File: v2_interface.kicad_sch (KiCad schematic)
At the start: 47 parts, among them J10 Power, J11 Vref_Select, J12 AUX_Select, J8 DE9_Socket, J9 DB25_Socket, Q1 2N7002K, Q2 2N7002K, U10 MCP1501-20xCH, U8 MCP4922, U9 MCP3424x-xSL

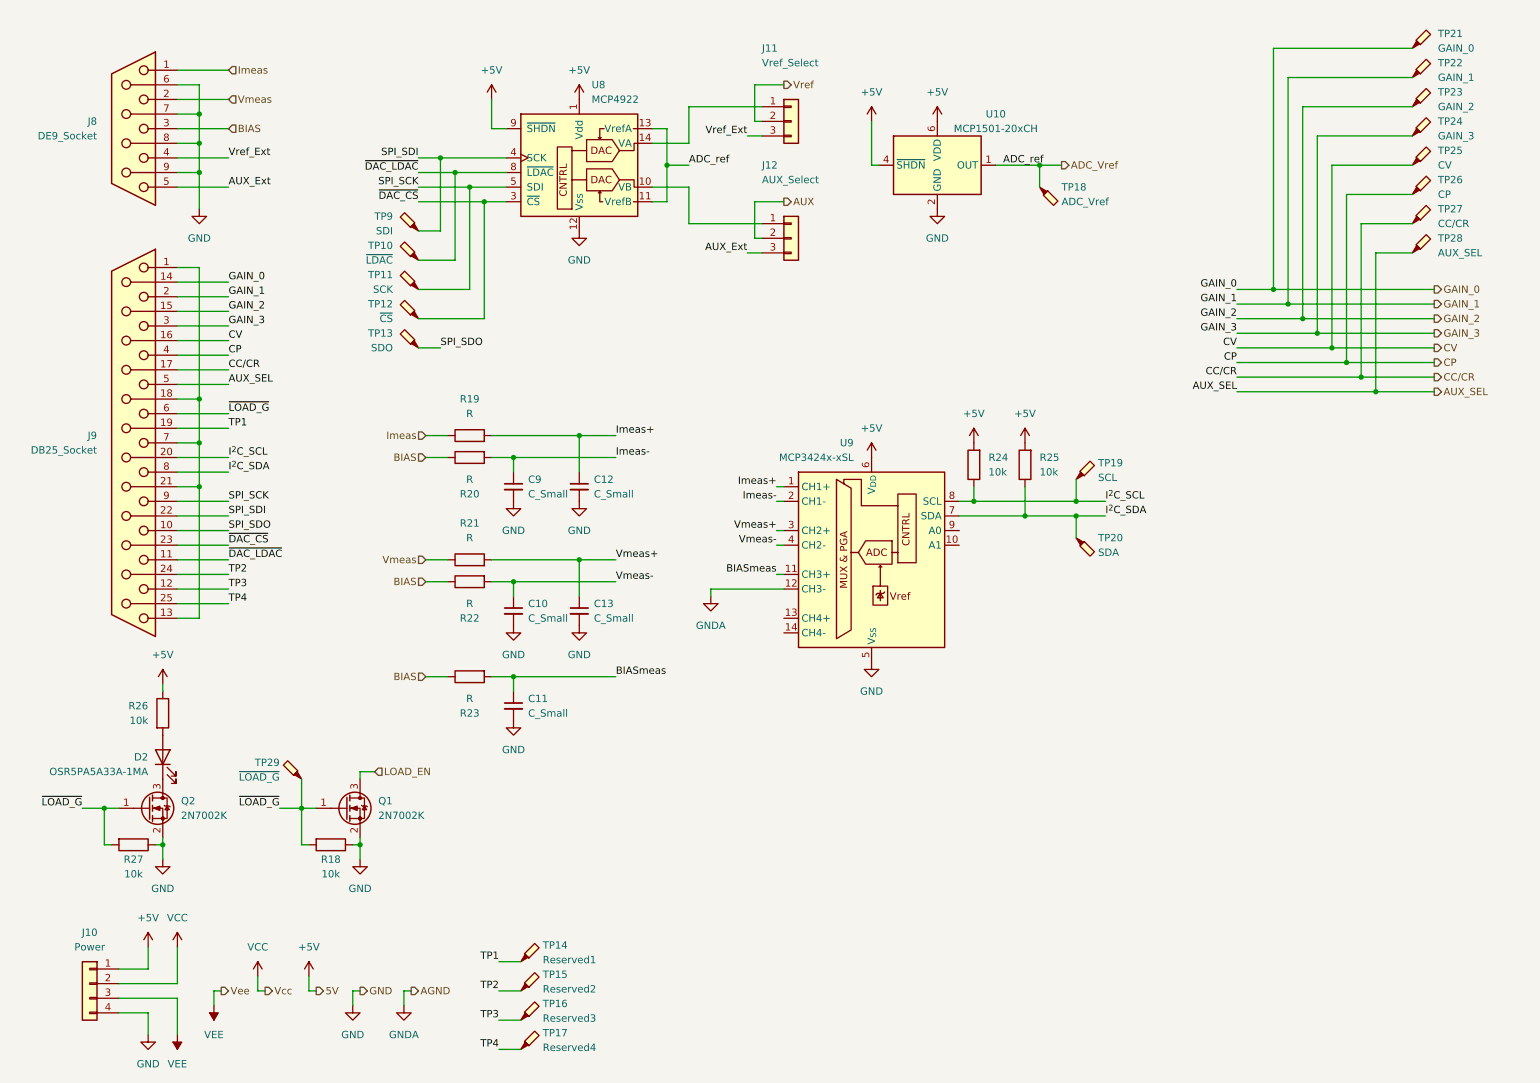
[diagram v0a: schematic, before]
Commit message: sims
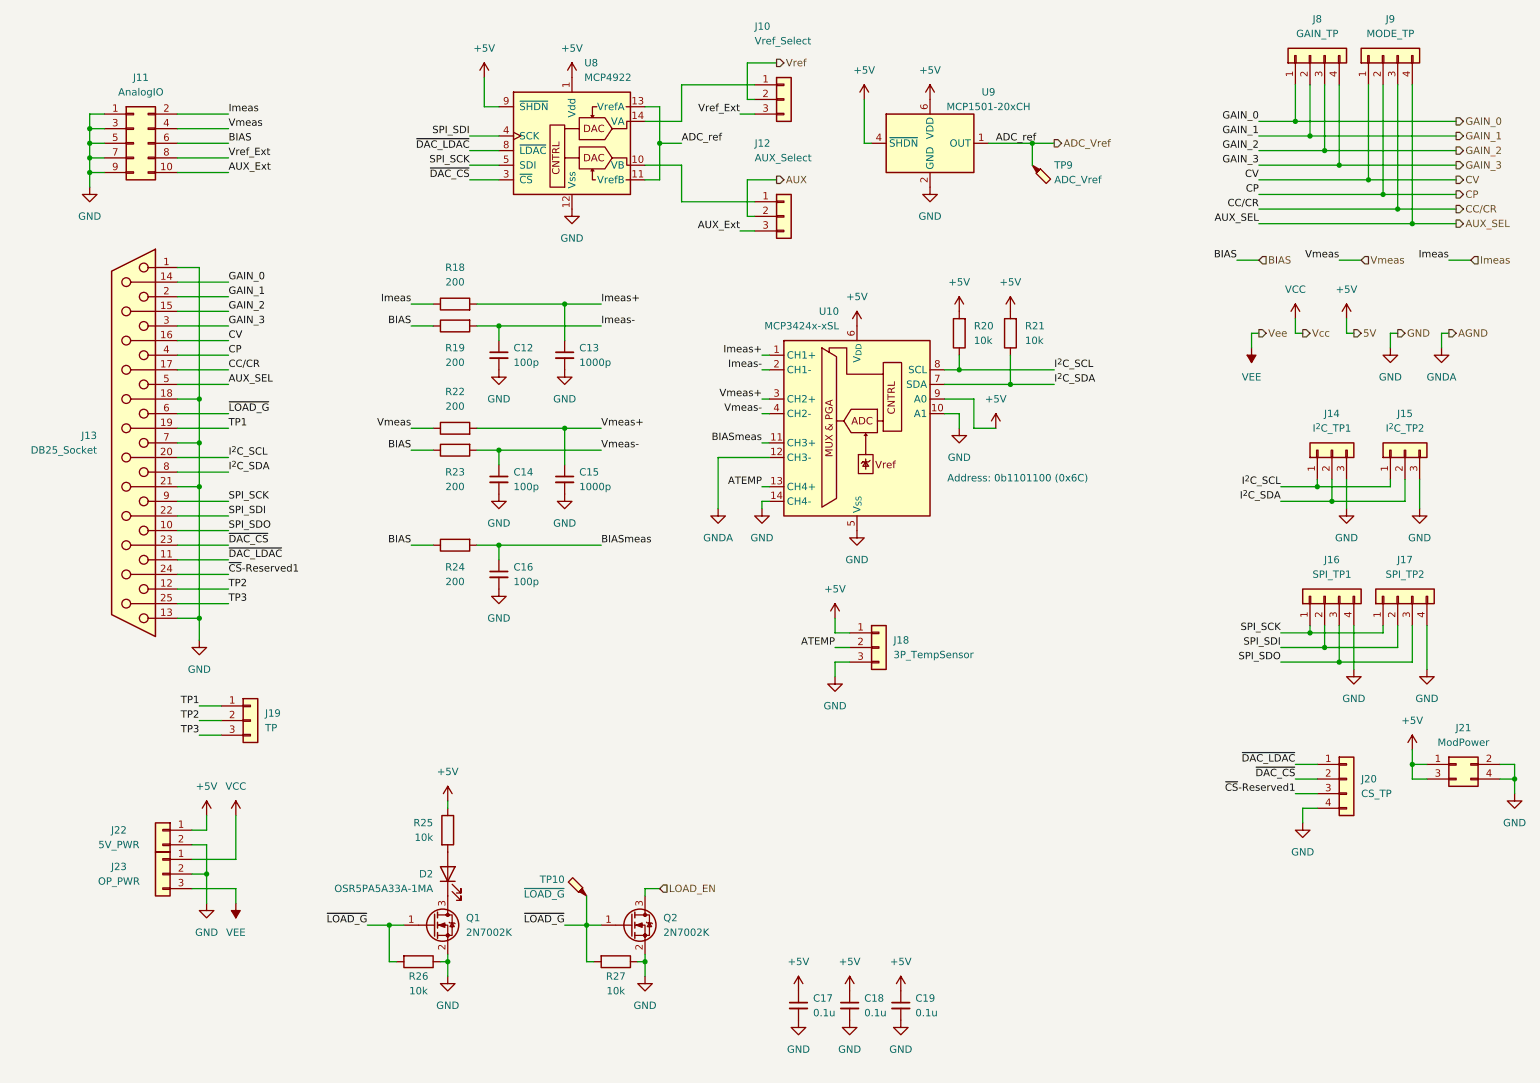
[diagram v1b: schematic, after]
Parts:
- removed J10: Power, AM_Conn_ScrewTerminal:TerminalReceptacle_1x04_P2.54mm, symbol Connector_Generic:Conn_01x04
- removed J8: DE9_Socket, AM_Conn_Dsub:Dsub-9P_2.77mm-2.84mm-8.08mmOffset, symbol Connector:DE9_Socket
- removed TP10: ~{LDAC}, symbol Connector:TestPoint_Probe
- removed TP11: SCK, symbol Connector:TestPoint_Probe
- removed TP12: ~{CS}, symbol Connector:TestPoint_Probe
- removed TP13: SDO, symbol Connector:TestPoint_Probe
- removed TP14: Reserved1, symbol Connector:TestPoint_Probe
- removed TP15: Reserved2, symbol Connector:TestPoint_Probe
- removed TP16: Reserved3, symbol Connector:TestPoint_Probe
- removed TP17: Reserved4, symbol Connector:TestPoint_Probe
- removed TP19: SCL, symbol Connector:TestPoint_Probe
- removed TP20: SDA, symbol Connector:TestPoint_Probe
- removed TP21: GAIN_0, symbol Connector:TestPoint_Probe
- removed TP22: GAIN_1, symbol Connector:TestPoint_Probe
- removed TP23: GAIN_2, symbol Connector:TestPoint_Probe
- removed TP24: GAIN_3, symbol Connector:TestPoint_Probe
- removed TP25: CV, symbol Connector:TestPoint_Probe
- removed TP26: CP, symbol Connector:TestPoint_Probe
- removed TP27: CC/CR, symbol Connector:TestPoint_Probe
- removed TP28: AUX_SEL, symbol Connector:TestPoint_Probe
- removed TP9: SDI, symbol Connector:TestPoint_Probe
- added C17, C18, C19: 0.1u, Capacitor_SMD:C_0603_1608Metric, symbol Device:C_Small
- added J11: AnalogIO, Connector_PinHeader_2.54mm:PinHeader_2x05_P2.54mm_Vertical, symbol Connector_Generic:Conn_02x05_Odd_Even
- added J14: I^{2}C_TP1, Connector_PinHeader_2.54mm:PinHeader_1x03_P2.54mm_Vertical, symbol Connector_Generic:Conn_01x03
- added J15: I^{2}C_TP2, Connector_PinHeader_2.54mm:PinHeader_1x03_P2.54mm_Vertical, symbol Connector_Generic:Conn_01x03
- added J16: SPI_TP1, Connector_PinHeader_2.54mm:PinHeader_1x04_P2.54mm_Vertical, symbol Connector_Generic:Conn_01x04
- added J17: SPI_TP2, Connector_PinHeader_2.54mm:PinHeader_1x04_P2.54mm_Vertical, symbol Connector_Generic:Conn_01x04
- added J18: 3P_TempSensor, Connector_PinSocket_2.54mm:PinSocket_1x03_P2.54mm_Vertical, symbol Connector_Generic:Conn_01x03
- added J19: TP, Connector_PinHeader_2.54mm:PinHeader_1x03_P2.54mm_Vertical, symbol Connector_Generic:Conn_01x03
- added J20: CS_TP, Connector_PinHeader_2.54mm:PinHeader_1x04_P2.54mm_Vertical, symbol Connector_Generic:Conn_01x04
- added J21: ModPower, Connector_PinHeader_2.00mm:PinHeader_2x02_P2.00mm_Vertical, symbol Connector_Generic:Conn_02x02_Odd_Even
- added J22: 5V_PWR, AM_Conn_ScrewTerminal:EurostylePluggable_1x02_P5.08mm, symbol Connector_Generic:Conn_01x02
- added J23: OP_PWR, AM_Conn_ScrewTerminal:EurostylePluggable_1x03_P5.08mm, symbol Connector_Generic:Conn_01x03
- added J8: GAIN_TP, Connector_PinHeader_2.54mm:PinHeader_1x04_P2.54mm_Vertical, symbol Connector_Generic:Conn_01x04
- added J9: MODE_TP, Connector_PinHeader_2.54mm:PinHeader_1x04_P2.54mm_Vertical, symbol Connector_Generic:Conn_01x04
- C12: renamed from C9; value C_Small -> 100p; footprint (none) -> Capacitor_SMD:C_0603_1608Metric
- C13: renamed from C12; value C_Small -> 1000p; footprint (none) -> Capacitor_SMD:C_0603_1608Metric
- C14: renamed from C10; value C_Small -> 100p; footprint (none) -> Capacitor_SMD:C_0603_1608Metric
- C15: renamed from C13; value C_Small -> 1000p; footprint (none) -> Capacitor_SMD:C_0603_1608Metric
- C16: renamed from C11; value C_Small -> 100p; footprint (none) -> Capacitor_SMD:C_0603_1608Metric
- R18: renamed from R19; value R -> 200; footprint (none) -> Resistor_SMD:R_0603_1608Metric
- R19: renamed from R20; value R -> 200; footprint (none) -> Resistor_SMD:R_0603_1608Metric
- R20: renamed from R24; footprint (none) -> Resistor_SMD:R_0603_1608Metric
- R21: renamed from R25; footprint (none) -> Resistor_SMD:R_0603_1608Metric
- R22: renamed from R21; value R -> 200; footprint (none) -> Resistor_SMD:R_0603_1608Metric
- R23: renamed from R22; value R -> 200; footprint (none) -> Resistor_SMD:R_0603_1608Metric
- R24: renamed from R23; value R -> 200; footprint (none) -> Resistor_SMD:R_0603_1608Metric
- R25: renamed from R26; footprint (none) -> Resistor_SMD:R_0603_1608Metric
- TP10: renamed from TP29; footprint (none) -> TestPoint:TestPoint_Loop_D2.50mm_Drill1.0mm
- TP9: renamed from TP18; footprint (none) -> TestPoint:TestPoint_Loop_D2.50mm_Drill1.0mm
- U10: renamed from U9; footprint Package_SO:SOIC-14_3.9x8.7mm_P1.27mm -> Package_DIP:DIP-14_W7.62mm
- U8: footprint (none) -> Package_DIP:DIP-14_W7.62mm
- renumbered J11 to J10, J9 to J13, Q2 to Q1, Q1 to Q2, R27 to R26, R18 to R27, U10 to U9
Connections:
- net TP4 is gone; now on net TP3: J13.25 (P25)
- net +5V: now also U10.9 (A0), C17.1, C18.1, C19.1, J18.1 (Pin_1), J21.1 (Pin_1), J21.3 (Pin_3), J22.1 (Pin_1)
- net AUX_Ext: now also J11.10 (Pin_10)
- net AUX_SEL: now also J9.4 (Pin_4)
- net BIAS: now also J11.6 (Pin_6)
- net CC/CR: now also J9.3 (Pin_3)
- net CP: now also J9.2 (Pin_2)
- net CV: now also J9.1 (Pin_1)
- net GAIN_0: now also J8.1 (Pin_1)
- net GAIN_1: now also J8.2 (Pin_2)
- net GAIN_2: now also J8.3 (Pin_3)
- net GAIN_3: now also J8.4 (Pin_4)
- net GND: now also J13.1, J13.13, J13.18 (P18), J13.21 (P21), J13.7, U10.10 (A1), U10.14 (CH4-), C17.2, C18.2, C19.2, J11.1 (Pin_1), J11.3 (Pin_3), J11.5 (Pin_5), J11.7 (Pin_7), J11.9 (Pin_9), J14.3 (Pin_3), J15.3 (Pin_3), J16.4 (Pin_4), J17.4 (Pin_4), J18.3 (Pin_3), J20.4 (Pin_4), J21.2 (Pin_2), J21.4 (Pin_4), J22.2 (Pin_2), J23.2 (Pin_2)
- net I^{2}C_SCL: now also J14.1 (Pin_1), J15.1 (Pin_1)
- net I^{2}C_SDA: now also J14.2 (Pin_2), J15.2 (Pin_2)
- net Imeas: now also J11.2 (Pin_2)
- net SPI_SCK: now also J16.1 (Pin_1), J17.1 (Pin_1)
- net SPI_SDI: now also J16.2 (Pin_2), J17.2 (Pin_2)
- net SPI_SDO: now also J16.3 (Pin_3), J17.3 (Pin_3)
- net TP1: now also J19.1 (Pin_1)
- net TP2: now also J13.12, J19.2 (Pin_2); no longer J13.24 (P24)
- net TP3: now also J19.3 (Pin_3); no longer J13.12
- net VCC: now also J23.1 (Pin_1)
- net VEE: now also J23.3 (Pin_3)
- net Vmeas: now also J11.4 (Pin_4)
- net Vref_Ext: now also J11.8 (Pin_8)
- net ~{DAC_CS}: now also J20.2 (Pin_2)
- net ~{DAC_LDAC}: now also J20.1 (Pin_1)
- net ATEMP: now reaches U10.13 (CH4+)
- net ATEMP: now also J18.2 (Pin_2)
- new net ~{CS}-Reserved1: J13.24 (P24), J20.3 (Pin_3)
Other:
- note added: "Address: 0b1101100 (0x6C)"
- moved on the sheet: C12, C13, C14, C15, C16, D2, J10, J12, Q1, Q2, R18, R19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
